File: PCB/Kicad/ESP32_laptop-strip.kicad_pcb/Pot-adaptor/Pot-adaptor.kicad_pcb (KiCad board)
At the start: 2 copper layers, 14.2 x 8.1 mm, 2 parts, among them J1 Conn_01x03_Socket

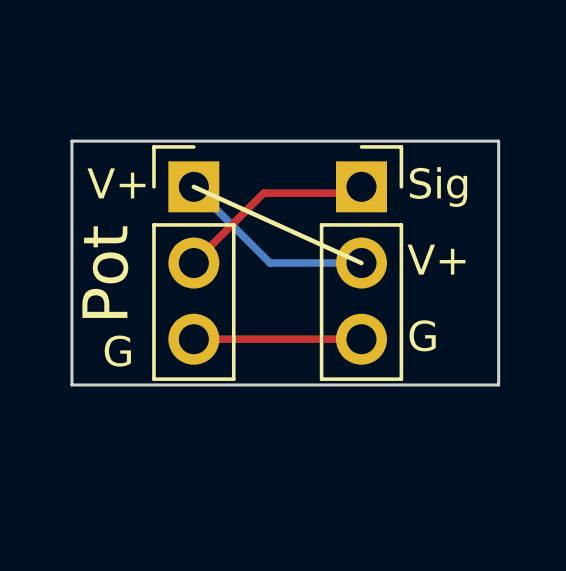
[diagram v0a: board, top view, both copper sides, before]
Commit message: July2026
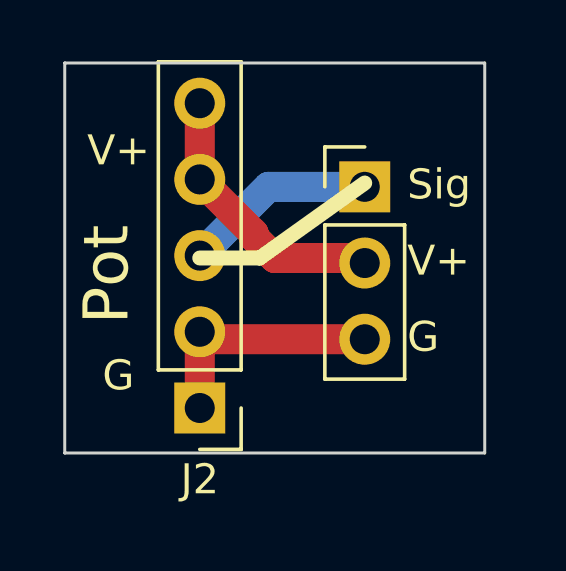
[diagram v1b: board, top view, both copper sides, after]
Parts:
- removed RV1: R_Potentiometer, Connector_PinSocket_2.54mm:PinSocket_1x03_P2.54mm_Vertical
- added J2: Conn_01x05_Socket, Connector_PinHeader_2.54mm:PinHeader_1x05_P2.54mm_Vertical, F.Cu at (146.5, 79.0)
- moved J1 5.70 mm to (152.0, 71.6)
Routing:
- net Net-(J1-Pin_2): track 6.64 -> 9.27 mm
- net Net-(J1-Pin_3): track 5.59 -> 8.14 mm
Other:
- board size 14.2 x 8.1 mm -> 14 x 13 mm
